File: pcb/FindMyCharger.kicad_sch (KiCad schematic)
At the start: 215 parts, among them IC1 CAV24C256WE-GT3, J1 USB_C_Receptacle, J3 Battery_Connector, J4 USB_C_Receptacle, Q1 Q_NMOS, Q2 Q_NMOS, Q3 Q_NMOS, Q4 Q_NMOS, Q5 Q_PMOS, Q6 Q_NMOS, Q7 Q_PMOS, Q8 Q_NMOS, Q9 Q_NMOS, SW1 SW_Push, SW2 SW_Push, SW3 SW_Push, U1 TPS25762DQRQLRQ1, U2 BQ25713RSNR, U3 BQ4050RSMR, U5 nRF54L10-QFXX, U6 TPS25730DREFR, Y1 32Mhz

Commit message: update
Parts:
- R62, R9: footprint (none) -> Resistor_SMD:R_0805_2012Metric; LCSC Part (none) -> C17414
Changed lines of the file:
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@@
 			)
 		)
-		(property "Footprint" ""
+		(property "Footprint" "Resistor_SMD:R_0805_2012Metric"
 			(at 108.458 533.4 90)
 			(hide yes)
@@
 			)
 		)
+		(property "LCSC Part" "C17414"
+			(at 106.68 533.4 0)
+			(hide yes)
+			(show_name no)
+			(do_not_autoplace no)
+			(effects
+				(font
+					(size 1.27 1.27)
+				)
+			)
+		)
 		(pin "1"
 		)
@@
 			)
 		)
-		(property "Footprint" ""
+		(property "Footprint" "Resistor_SMD:R_0805_2012Metric"
 			(at 99.568 530.86 90)
 			(hide yes)
@@
 			(at 97.79 530.86 0)
 			(hide yes)
+			(show_name no)
+			(do_not_autoplace no)
+			(effects
+				(font
+					(size 1.27 1.27)
+				)
+			)
+		)
+		(property "LCSC Part" "C17414"
+			(at 97.79 530.86 0)
+			(hide yes)

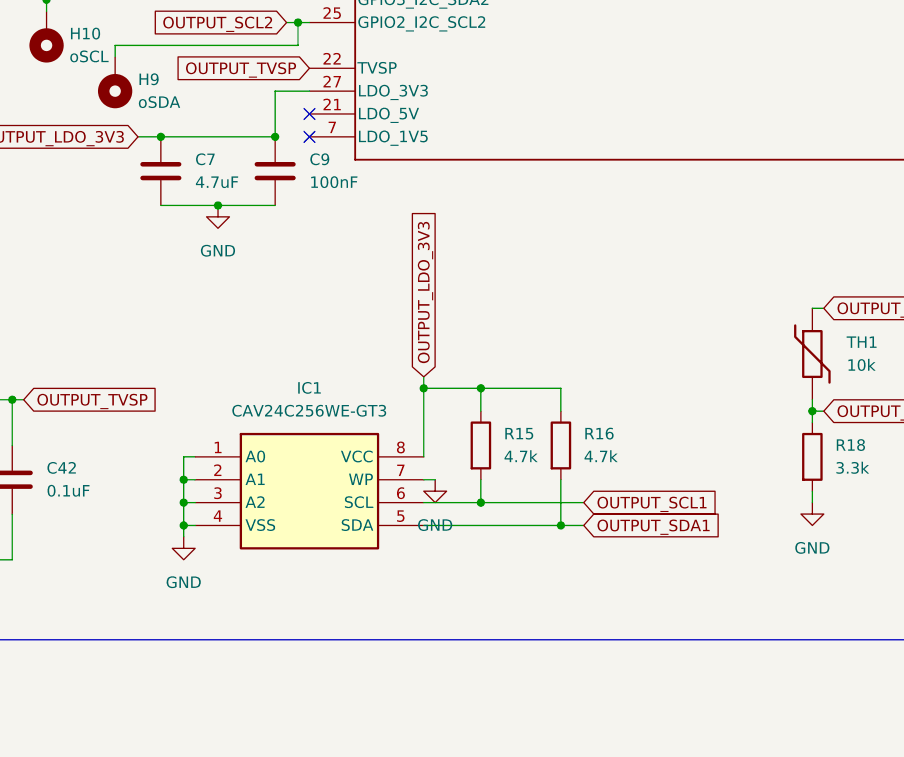
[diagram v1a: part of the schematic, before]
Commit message: a
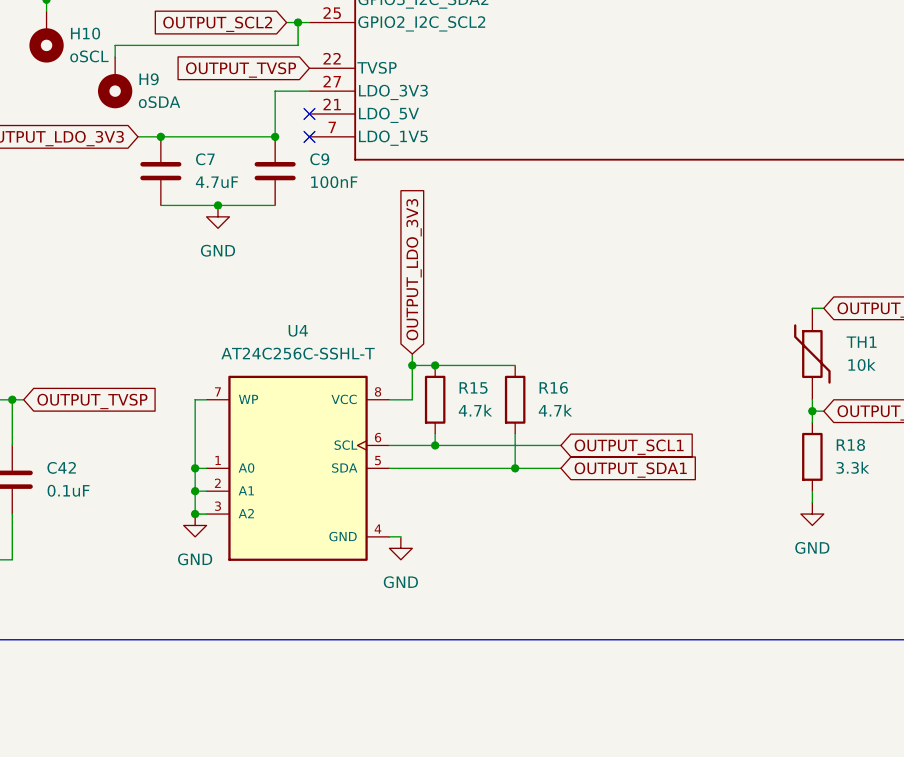
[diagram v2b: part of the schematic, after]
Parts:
- removed IC1: CAV24C256WE-GT3, symbol CAV24C256WE-GT3:CAV24C256WE-GT3
- added U4: AT24C256C-SSHL-T, AT24C256C-SSHL-T:SOIC127P600X175-8N, symbol AT24C256C-SSHL-T:AT24C256C-SSHL-T
- Q1, Q2, Q3, Q4: footprint footprints:CSD17308Q3 -> (none); MPN CSD17308Q3 -> (none)
- Q5: footprint Package_TO_SOT_SMD:SOT-23 -> (none); MPN CSD25404Q3 -> (none)
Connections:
- net GND: now also U4.1 (A0), U4.2 (A1), U4.3 (A2), U4.4 (GND), U4.7 (WP)
- net OUTPUT_LDO_3V3: now also U4.8 (VCC)
- net OUTPUT_SCL1: now also U4.6 (SCL)
- net OUTPUT_SDA1: now also U4.5 (SDA)
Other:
- moved on the sheet: R15, R16
